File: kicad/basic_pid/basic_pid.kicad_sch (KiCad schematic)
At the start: 67 parts, among them J1 Input A, J2 Input B / Setpoint, J3 Output, J4 Output, SW1 SW_DPDT_x2, SW2 SW_DPDT_x2, SW3 SW_SPDT, SW4 SW_SP4T, SW5 SW_SPDT, SW6 SW_SP4T, SW7 SW_SP4T, SW8 SW_SP4T, SW9 SW_SP4T, U1 LM4040LP-5, U10 OPA189, U11 OPA189, U12 OPA189, U13 BUF634A, U2 LM4040LP-5, U3 LT1167, U4 LT1167, U5 OPA189, U6 OPA189, U7 OPA189, U8 BUF634A, U9 OPA189

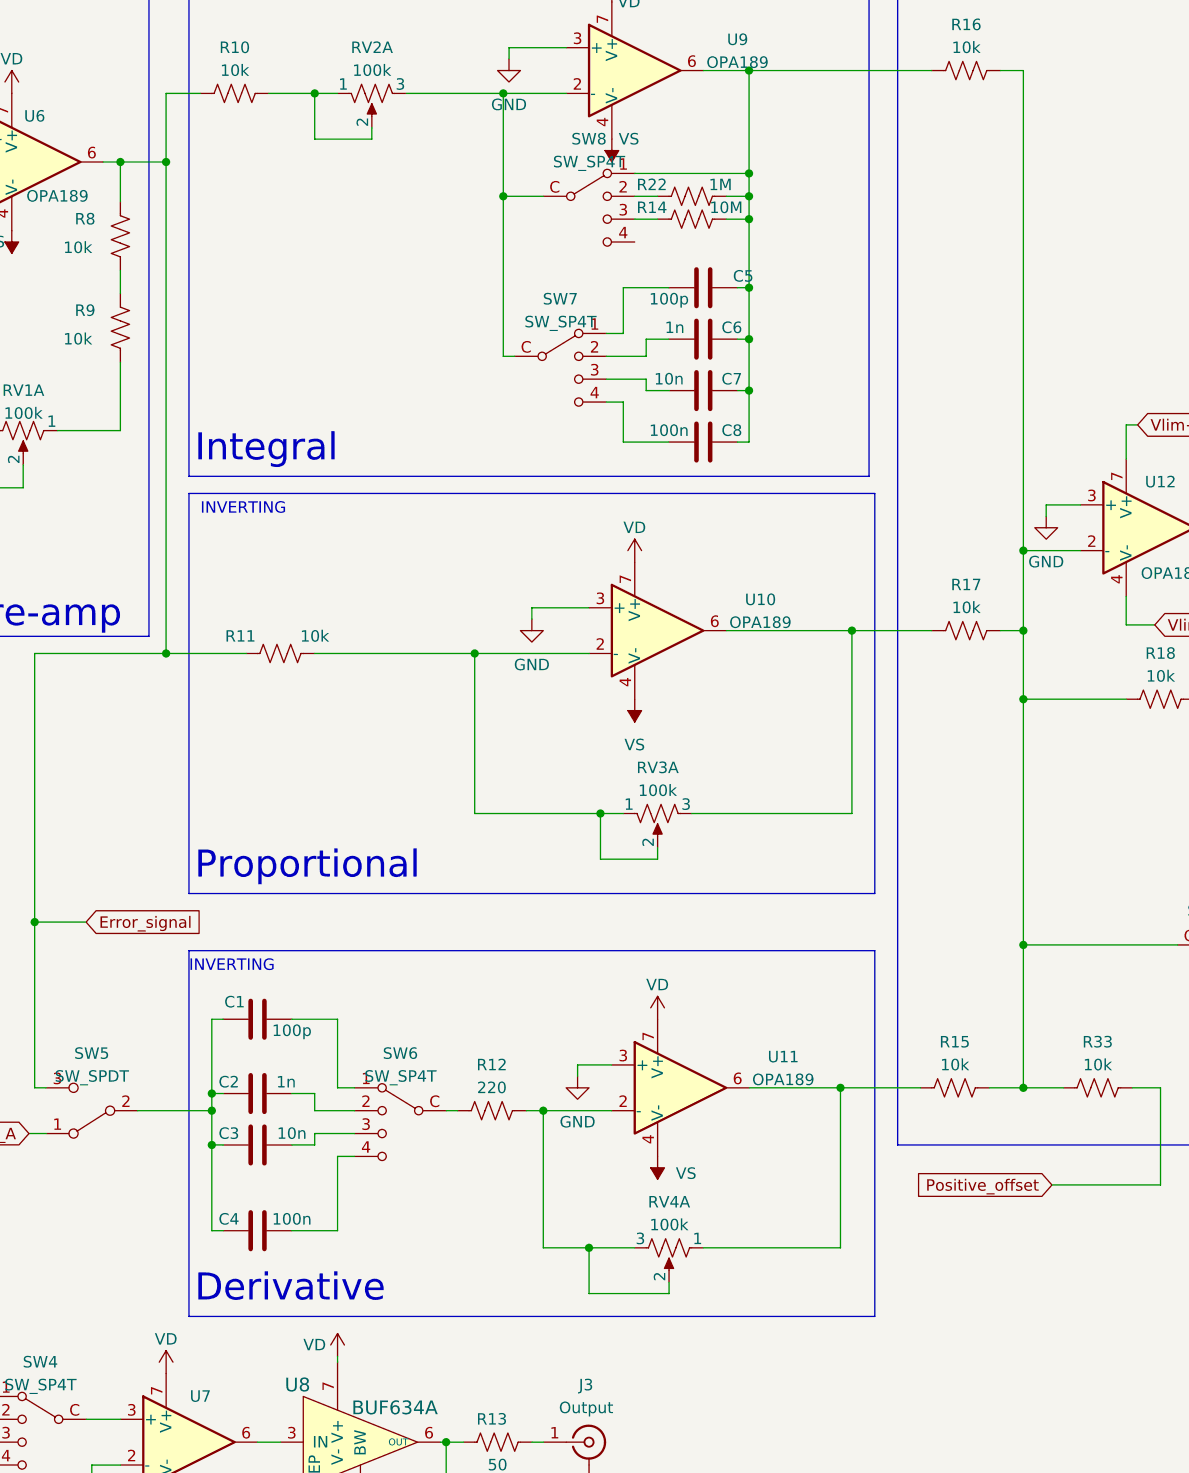
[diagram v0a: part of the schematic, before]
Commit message: This contains ideas for a high-speed design
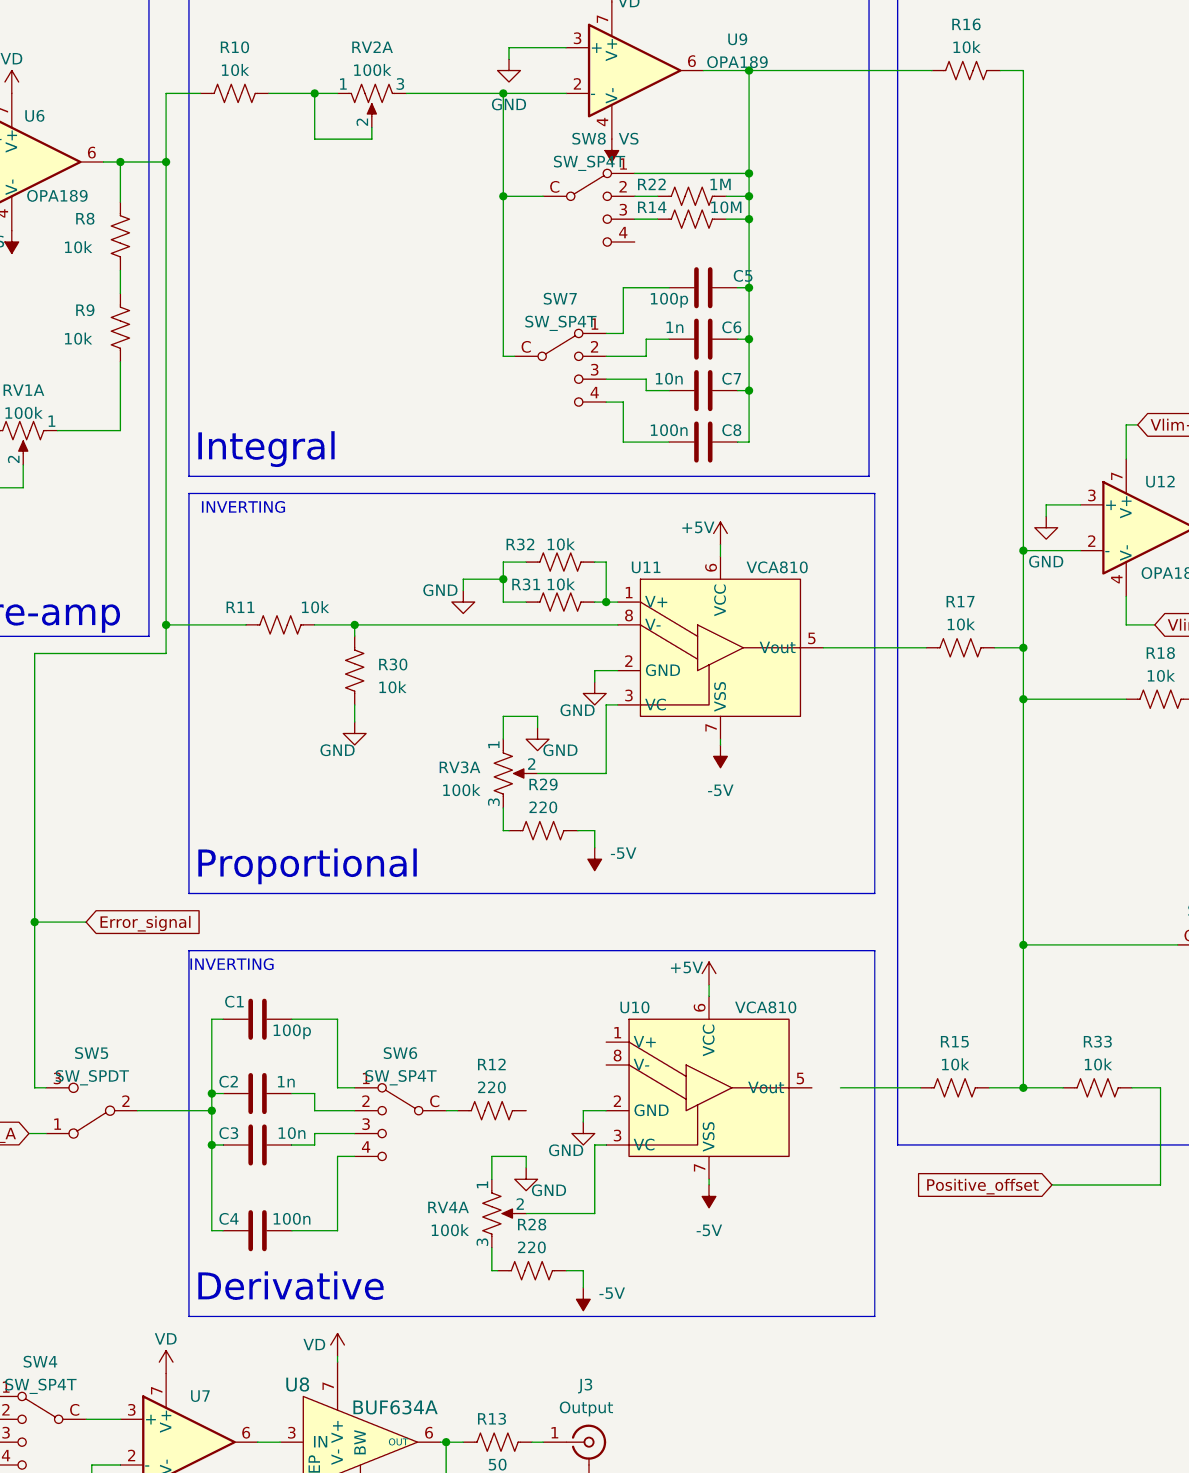
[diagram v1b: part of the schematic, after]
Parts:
- removed U10, U11: OPA189, Package_SO:SOIC-8_3.9x4.9mm_P1.27mm, symbol Amplifier_Operational:OPA330xxD
- added R28, R29: 220, Resistor_SMD:R_0805_2012Metric, symbol Device:R_US
- added R30, R31, R32: 10k, Resistor_SMD:R_0805_2012Metric, symbol Device:R_US
- added U10, U11: VCA810, Package_SO:SOIC-8_3.9x4.9mm_P1.27mm, symbol local_lib:VCA810
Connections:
- net GND: now also RV3.1, RV4.1, R30.1, R31.2, R32.2, U10.2 (GND), U11.2 (GND)
- net at R15.1: no longer RV4.1
- net at R17.1: now also U11.5 (Vout); no longer RV3.3
- new net: R31.1, R32.1, U11.1 (V+)
- new net: RV3.2, U11.3 (VC)
- new net: R29.2, RV3.3
- new net: RV4.2, U10.3 (VC)
- new net: R28.2, RV4.3
- new net: R11.2, R30.2, U11.8 (V-)
- new net +5V: U10.6 (VCC), U11.6 (VCC)
- new net -5V: R28.1, R29.1, U10.7 (VSS), U11.7 (VSS)
- now unconnected: R12.2
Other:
- moved on the sheet: R11, R17, RV4A
